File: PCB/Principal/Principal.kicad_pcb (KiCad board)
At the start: 2 copper layers, 128.3 x 134.6 mm, 17 parts, among them J1 STM32_P1, J2 STM32_P2, J3 Sensor_Golpes, J4 Teclado, J5 Sensor_Unidades, J6 Display_16x2, J7 Lector_RFID, J8 IN_Alimentación

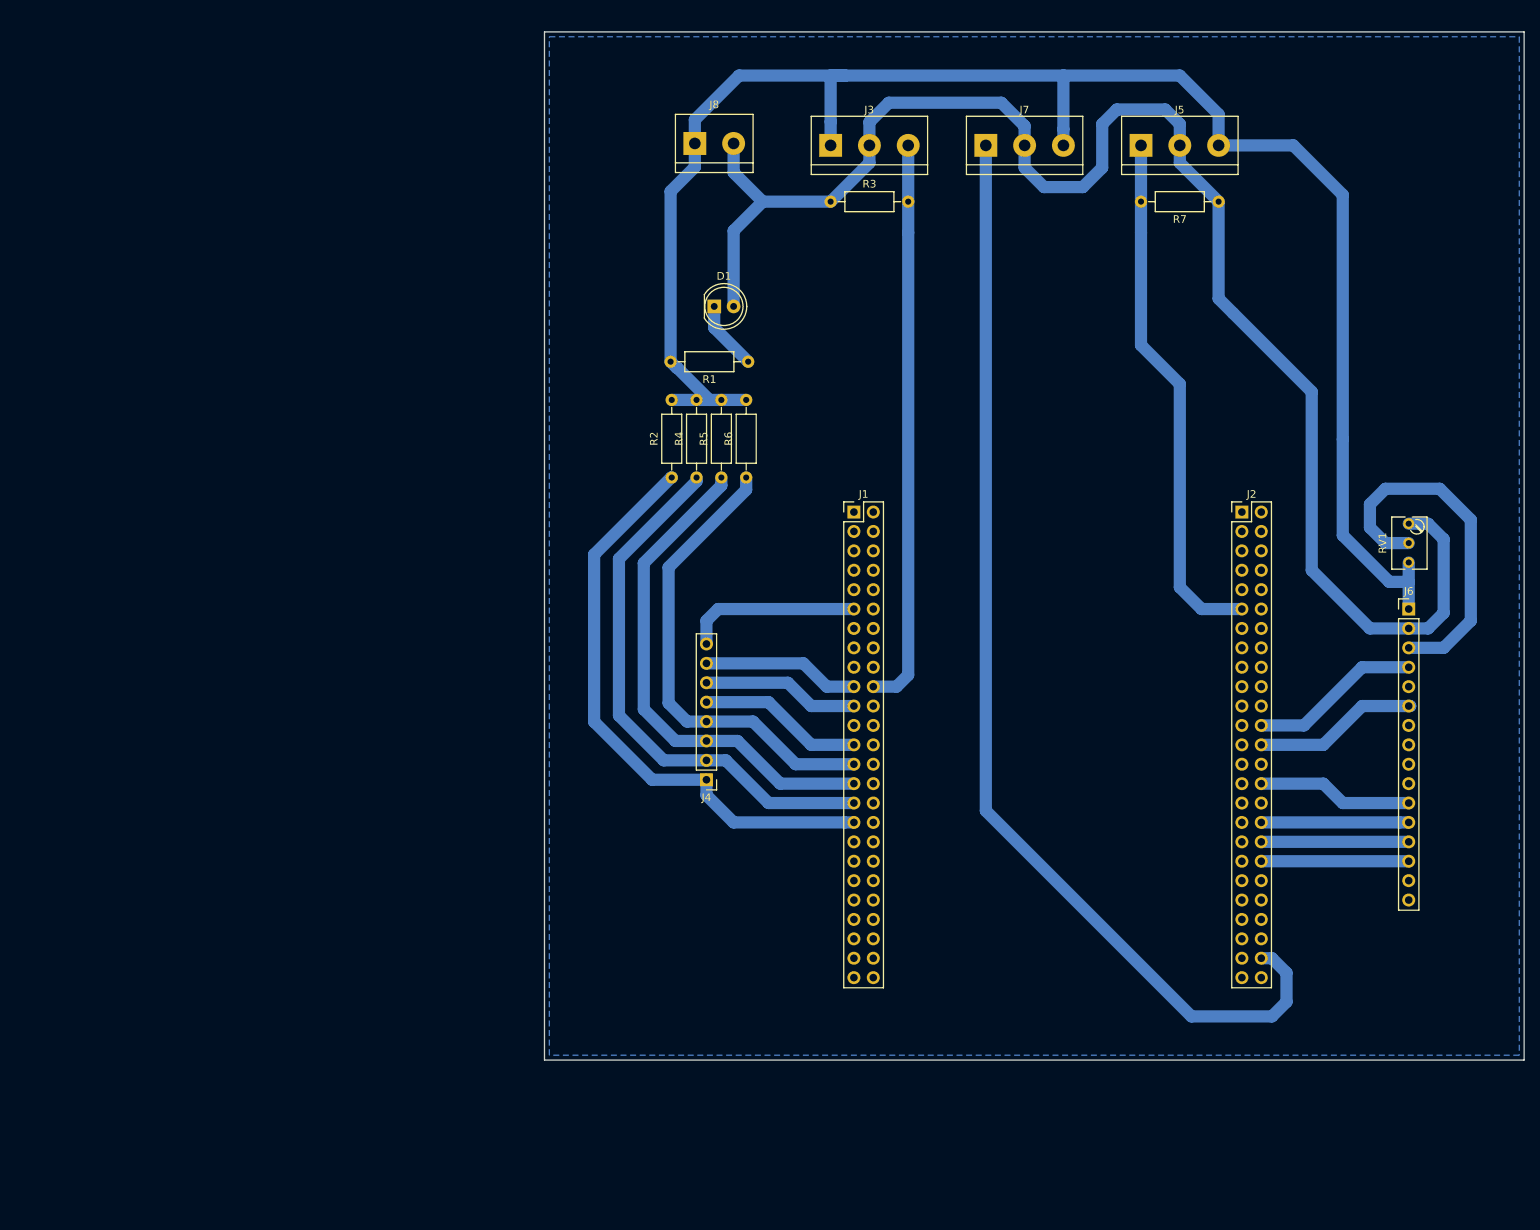
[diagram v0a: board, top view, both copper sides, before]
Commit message: Fin PCB re piola
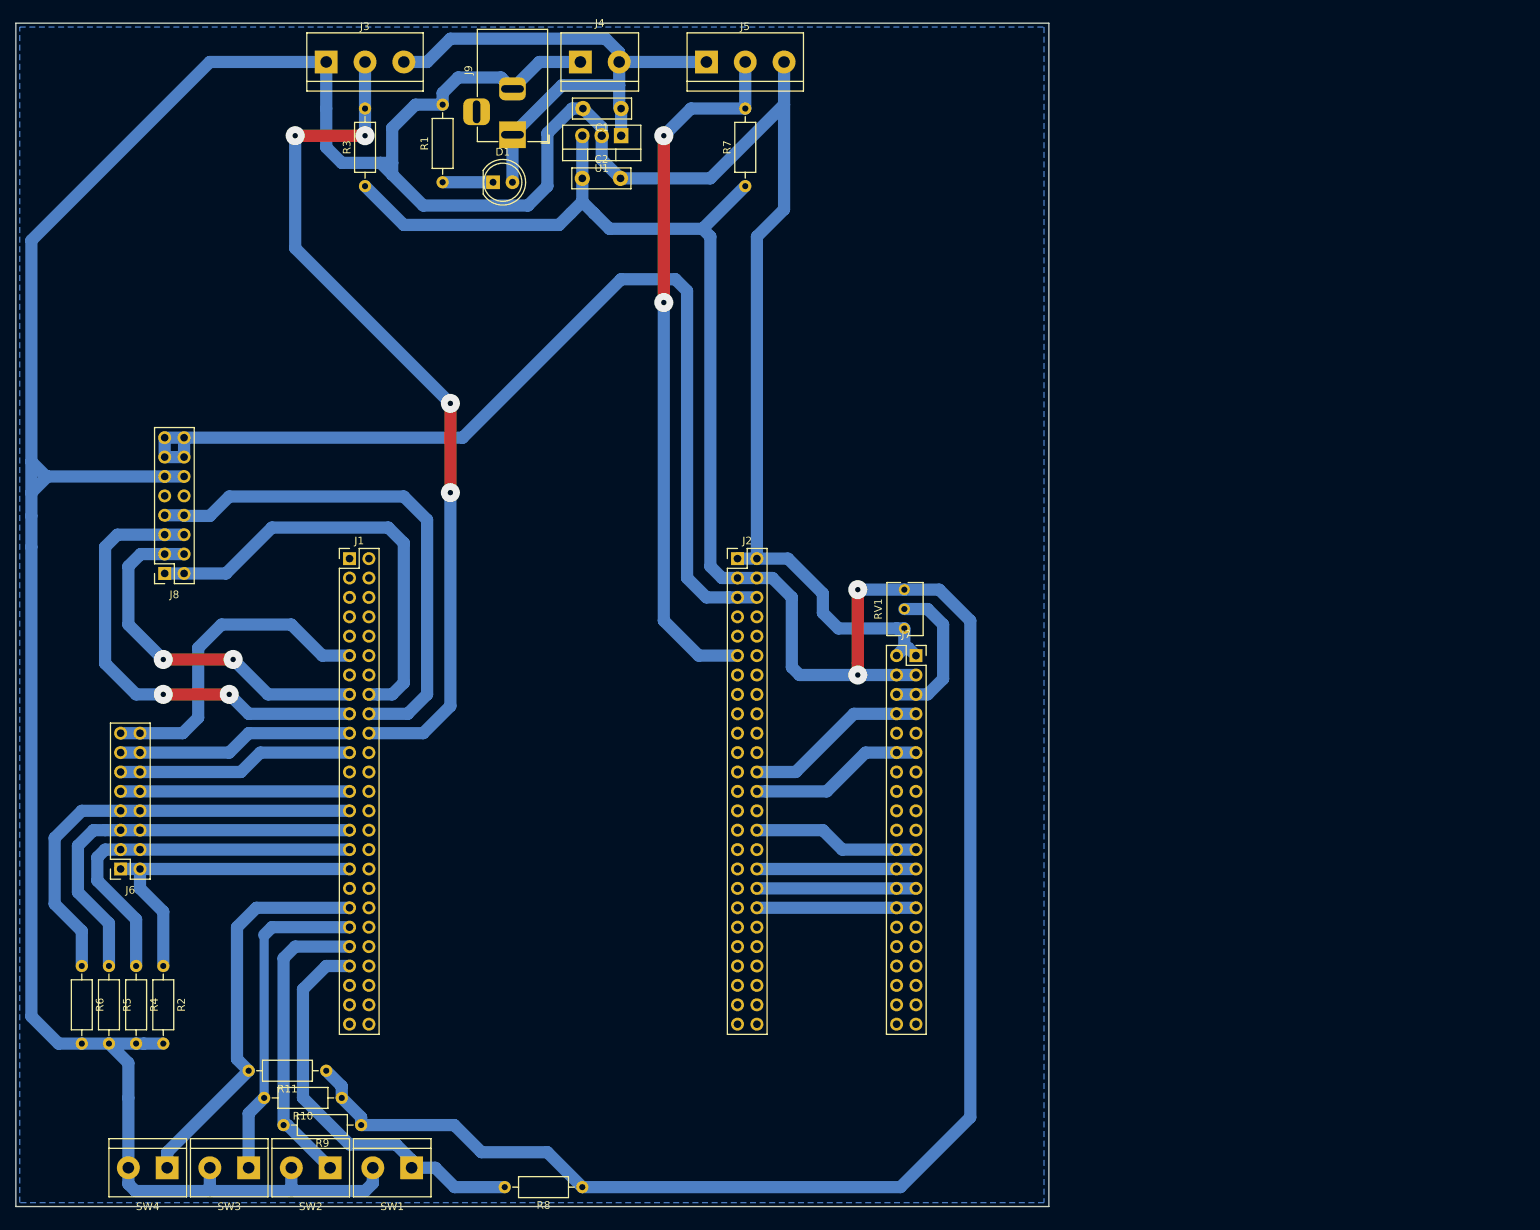
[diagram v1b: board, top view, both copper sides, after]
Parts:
- added C1: 330n, Capacitor_THT:C_Disc_D7.5mm_W2.5mm_P5.00mm, F.Cu at (91.9, 28.4)
- added C2: 100n, Capacitor_THT:C_Disc_D7.5mm_W2.5mm_P5.00mm, F.Cu at (86.9, 37.6)
- added J9: Jack-DC, Connector_BarrelJack:BarrelJack_Horizontal, F.Cu at (77.7, 31.9)
- added R10: 4,7k, Resistor_THT:R_Axial_DIN0207_L6.3mm_D2.5mm_P10.16mm_Horizontal, F.Cu at (55.4, 158.0)
- added R11: 4,7k, Resistor_THT:R_Axial_DIN0207_L6.3mm_D2.5mm_P10.16mm_Horizontal, F.Cu at (53.3, 154.4)
- added R8: 4,7k, Resistor_THT:R_Axial_DIN0207_L6.3mm_D2.5mm_P10.16mm_Horizontal, F.Cu at (86.9, 169.7)
- added R9: 4,7k, Resistor_THT:R_Axial_DIN0207_L6.3mm_D2.5mm_P10.16mm_Horizontal, F.Cu at (57.9, 161.5)
- added SW1: InputPullUp1, TerminalBlock:TerminalBlock_bornier-2_P5.08mm, F.Cu at (64.5, 167.1)
- added SW2: InputPullUp2, TerminalBlock:TerminalBlock_bornier-2_P5.08mm, F.Cu at (53.8, 167.1)
- added SW3: InputPullUp3, TerminalBlock:TerminalBlock_bornier-2_P5.08mm, F.Cu at (43.2, 167.1)
- added SW4: InputPullUp4, TerminalBlock:TerminalBlock_bornier-2_P5.08mm, F.Cu at (32.5, 167.1)
- added U1: LM7805, Package_TO_SOT_THT:TO-220-3_Vertical, F.Cu at (91.9, 32.0)
- D1: footprint LEDs:LED_D5.0mm -> LED_THT:LED_D5.0mm
- J1, J2: footprint Pin_Headers:Pin_Header_Straight_2x25_Pitch2.54mm -> Connector_PinHeader_2.54mm:PinHeader_2x25_P2.54mm_Vertical
- J3, J5: footprint Connectors_Terminal_Blocks:TerminalBlock_bornier-3_P5.08mm -> TerminalBlock:TerminalBlock_bornier-3_P5.08mm
- J4: value Teclado -> Fuente; footprint Pin_Headers:Pin_Header_Straight_1x08_Pitch2.54mm -> TerminalBlock:TerminalBlock_bornier-2_P5.08mm
- J6: value Display_16x2 -> Conn_Teclado; footprint Pin_Headers:Pin_Header_Straight_1x16_Pitch2.54mm -> Connector_PinSocket_2.54mm:PinSocket_2x08_P2.54mm_Vertical
- J7: value Lector_RFID -> Conn_Display; footprint Connectors_Terminal_Blocks:TerminalBlock_bornier-3_P5.08mm -> Connector_PinSocket_2.54mm:PinSocket_2x20_P2.54mm_Vertical
- J8: value IN_Alimentación -> Conn_RFID; footprint Connectors_Terminal_Blocks:TerminalBlock_bornier-2_P5.08mm -> Connector_PinSocket_2.54mm:PinSocket_2x08_P2.54mm_Vertical
- R1: value 330 -> 680; footprint Resistors_THT:R_Axial_DIN0207_L6.3mm_D2.5mm_P10.16mm_Horizontal -> Resistor_THT:R_Axial_DIN0207_L6.3mm_D2.5mm_P10.16mm_Horizontal
- R2, R3, R4, R5, R6, R7: footprint Resistors_THT:R_Axial_DIN0207_L6.3mm_D2.5mm_P10.16mm_Horizontal -> Resistor_THT:R_Axial_DIN0207_L6.3mm_D2.5mm_P10.16mm_Horizontal
- RV1: footprint Potentiometers:Potentiometer_Trimmer_Bourns_3266Y -> Potentiometer_THT:Potentiometer_Bourns_3266Y_Vertical
- moved J6 172.1 mm to (26.4, 128.0), turned to 180 degrees
- moved R6 108.0 mm to (21.3, 140.7), turned to 270 degrees
- moved R5 102.6 mm to (24.9, 140.7), turned to 270 degrees
- moved R4 97.3 mm to (28.4, 140.7), turned to 270 degrees
- moved J4 95.4 mm to (86.6, 22.4), turned to 0 degrees
- moved R2 92.3 mm to (32.0, 140.7), turned to 270 degrees
- moved J8 89.4 mm to (32.2, 89.3), turned to 180 degrees
- moved J7 67.4 mm to (130.6, 100.1)
- moved J3 66.9 mm to (53.3, 22.4)
- moved RV1 66.6 mm to (129.0, 91.4)
- moved J2 66.3 mm to (107.2, 87.4)
- moved J1 66.3 mm to (56.4, 87.4)
- moved R7 62.0 mm to (108.2, 38.6), turned to 90 degrees
- moved R3 61.0 mm to (58.4, 38.6), turned to 90 degrees
- moved J5 57.9 mm to (103.1, 22.4)
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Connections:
- D1 pad 2: +5V -> /9V
- J1 pad 15: Net-(J1-Pad15) -> PA5
- J1 pad 16: Net-(J1-Pad16) -> PA4
- J1 pad 17: Net-(J1-Pad17) -> PA7
- J1 pad 18: Net-(J1-Pad18) -> PA6
- J2 pad 1: Net-(J2-Pad1) -> GND
- J2 pad 2: Net-(J2-Pad2) -> GND
- J2 pad 3: Net-(J2-Pad3) -> 5V
- J2 pad 4: Net-(J2-Pad4) -> 5V
- J2 pad 5: Net-(J2-Pad5) -> 3V
- J2 pad 6: Net-(J2-Pad6) -> 3V
- J3 pad 3: +5V -> /9V
- J4 pad 1: Net-(J1-Pad33) -> GND
- J4 pad 2: Net-(J1-Pad31) -> /9V
- J5 pad 1: +5V -> /9V
- J6 pad 1: GND -> Net-(J1-Pad33)
- J6 pad 10: Net-(J6-Pad10) -> Net-(J1-Pad25)
- J6 pad 11: Net-(J2-Pad30) -> Net-(J1-Pad21)
- J6 pad 12: Net-(J2-Pad34) -> Net-(J1-Pad21)
- J6 pad 13: Net-(J2-Pad36) -> Net-(J1-Pad19)
- J6 pad 14: Net-(J2-Pad38) -> Net-(J1-Pad19)
- J6 pad 15: Net-(J6-Pad15) -> Net-(J1-Pad11)
- J6 pad 16: Net-(J6-Pad16) -> Net-(J1-Pad11)
- J6 pad 2: +5V -> Net-(J1-Pad33)
- J6 pad 3: Net-(J6-Pad3) -> Net-(J1-Pad31)
- J6 pad 4: Net-(J2-Pad24) -> Net-(J1-Pad31)
- J6 pad 5: Net-(J6-Pad5) -> Net-(J1-Pad29)
- J6 pad 6: Net-(J2-Pad26) -> Net-(J1-Pad29)
- J6 pad 7: Net-(J6-Pad7) -> Net-(J1-Pad27)
- J6 pad 8: Net-(J6-Pad8) -> Net-(J1-Pad27)
- J6 pad 9: Net-(J6-Pad9) -> Net-(J1-Pad25)
- J7 pad 1: +5V -> GND
- J7 pad 2: Net-(J2-Pad48) -> GND
- J7 pad 3: GND -> 5V
- J8 pad 1: GND -> PA4
- J8 pad 2: +5V -> PA4
- R3 pad 1: +5V -> 5V
- R7 pad 1: +5V -> 5V
- RV1 pad 1: +5V -> 5V
- RV1 pad 2: Net-(J6-Pad3) -> Net-(J7-Pad5)
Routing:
- net 5V: track 0.00 -> 336.9 mm, vias 0 -> 2
- net GND: track 228.0 -> 484.0 mm
- net +5V: track 205.6 -> 0.00 mm
- net Net-(J2-Pad48): track 146.3 -> 0.00 mm
- net 3V: track 0.00 -> 133.0 mm
- net /9V: track 0.00 -> 75.5 mm
- net PA6: track 0.00 -> 68.2 mm
- net PA7: track 0.00 -> 61.0 mm, vias 0 -> 2
- net PA4: track 0.00 -> 58.1 mm
- net Net-(J1-Pad43): track 0.00 -> 53.4 mm
- net Net-(J1-Pad37): track 0.00 -> 52.3 mm
- net PA5: track 0.00 -> 48.3 mm, vias 0 -> 2
- net Net-(J6-Pad3): track 47.5 -> 0.00 mm
- net Net-(J1-Pad39): track 0.00 -> 42.9 mm
- net Net-(J1-Pad41): track 0.00 -> 40.0 mm
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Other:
- board size 128.3 x 134.6 mm -> 135.3 x 154.9 mm
- rule trace_min: 0.2 -> 0.3
